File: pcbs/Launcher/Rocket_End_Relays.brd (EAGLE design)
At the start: 100 x 80 mm, 39 parts, among them IC2 LM2576T-ADJ, K4 LD105, K5 LD105, K6 LD105, K7 LD105, T1 BC547, T2 BC547, T3 BC547, T4 BC547, T5 BC547, U1 ARDUINO-MEGAPRO-5V, X1 1751248, X2 22-23-2041, X3 22-23-2021, X4 1751248

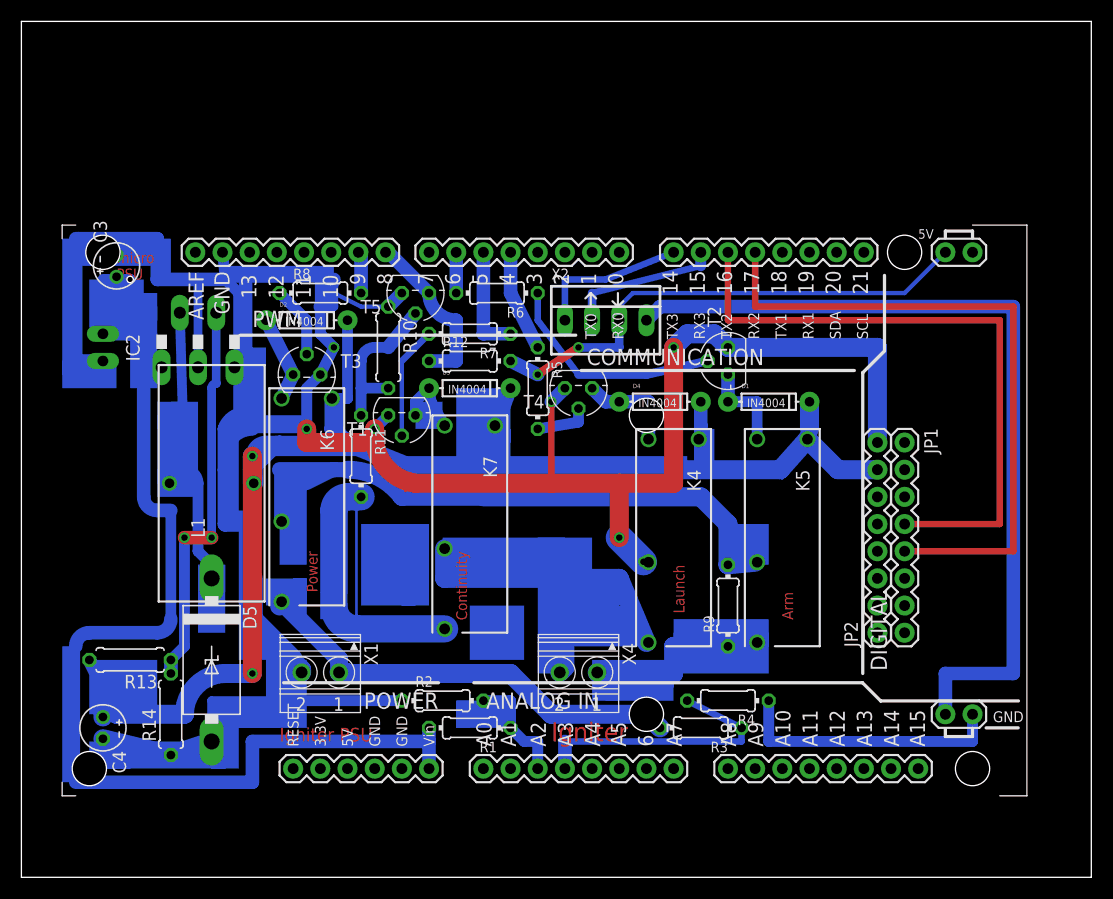
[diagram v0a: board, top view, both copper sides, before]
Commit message: * various updates to pcbs
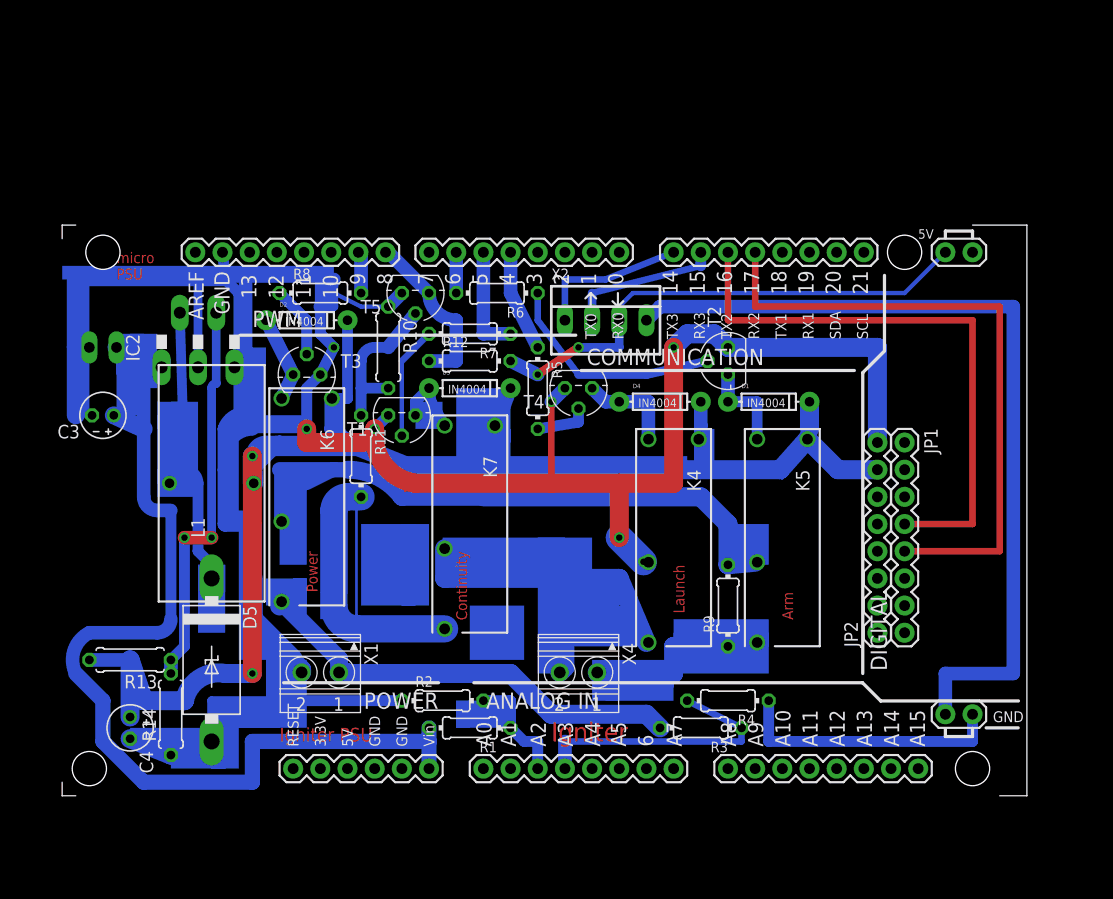
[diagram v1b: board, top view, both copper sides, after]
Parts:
- moved C3 14.0 mm to (7.62, 43.2), turned to 180 degrees
- moved C4 2.54 mm to (10.2, 14.0)
- turned X3 to 0 degrees
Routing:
- net VCC: track 112.1 -> 95.0 mm
- net N$33: track 282.6 -> 271.5 mm
- net N$1: track 59.7 -> 54.6 mm
- net N$2: track 62.2 -> 59.7 mm
- net N$5: track 161.0 -> 162.4 mm
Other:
- board outline removed
